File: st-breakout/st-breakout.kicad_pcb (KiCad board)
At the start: 2 copper layers, 72 x 51 mm, 35 parts, among them J1 SPI, J2 SWD, J3 USB4085-GF-A_REVB, J4 USART, SW1 SW_SPDT, U1 AP63203WU, U2 STM32F070F6Px, Y1 16 MHz

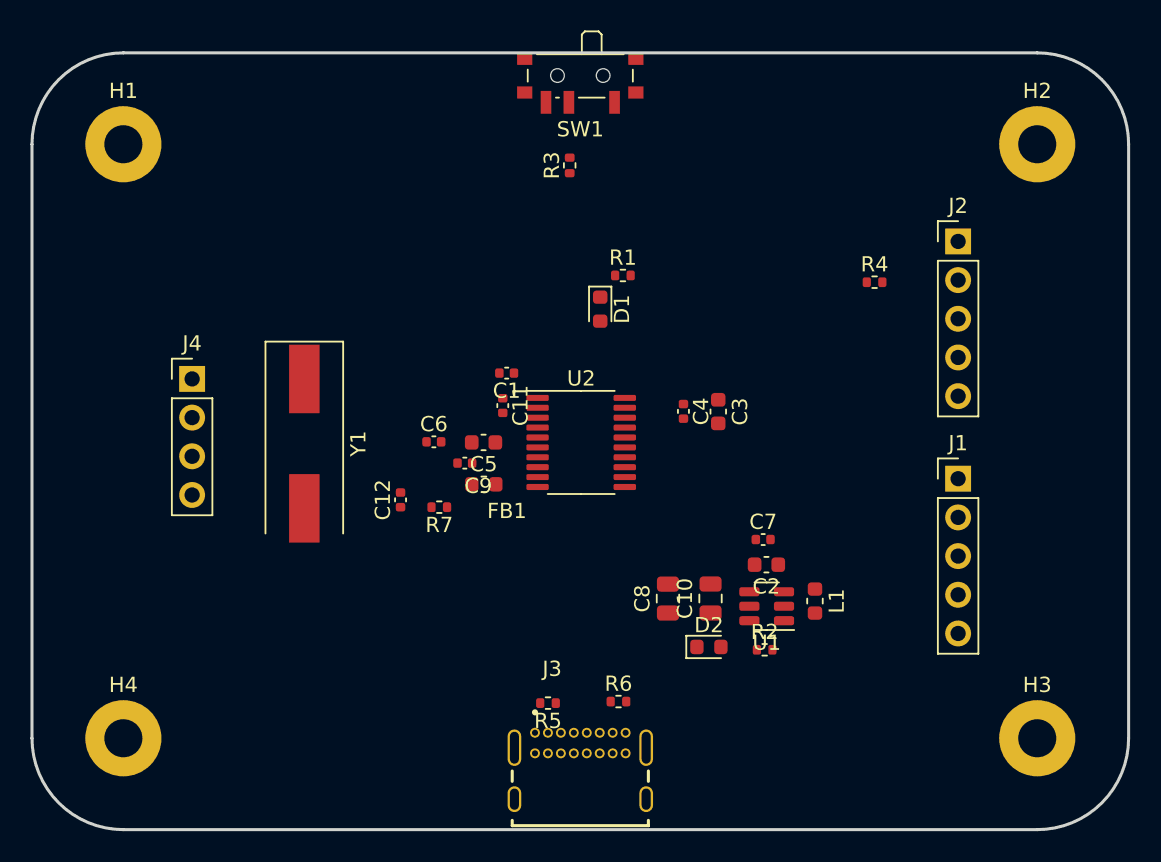
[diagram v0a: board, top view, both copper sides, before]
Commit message: routing and gerber
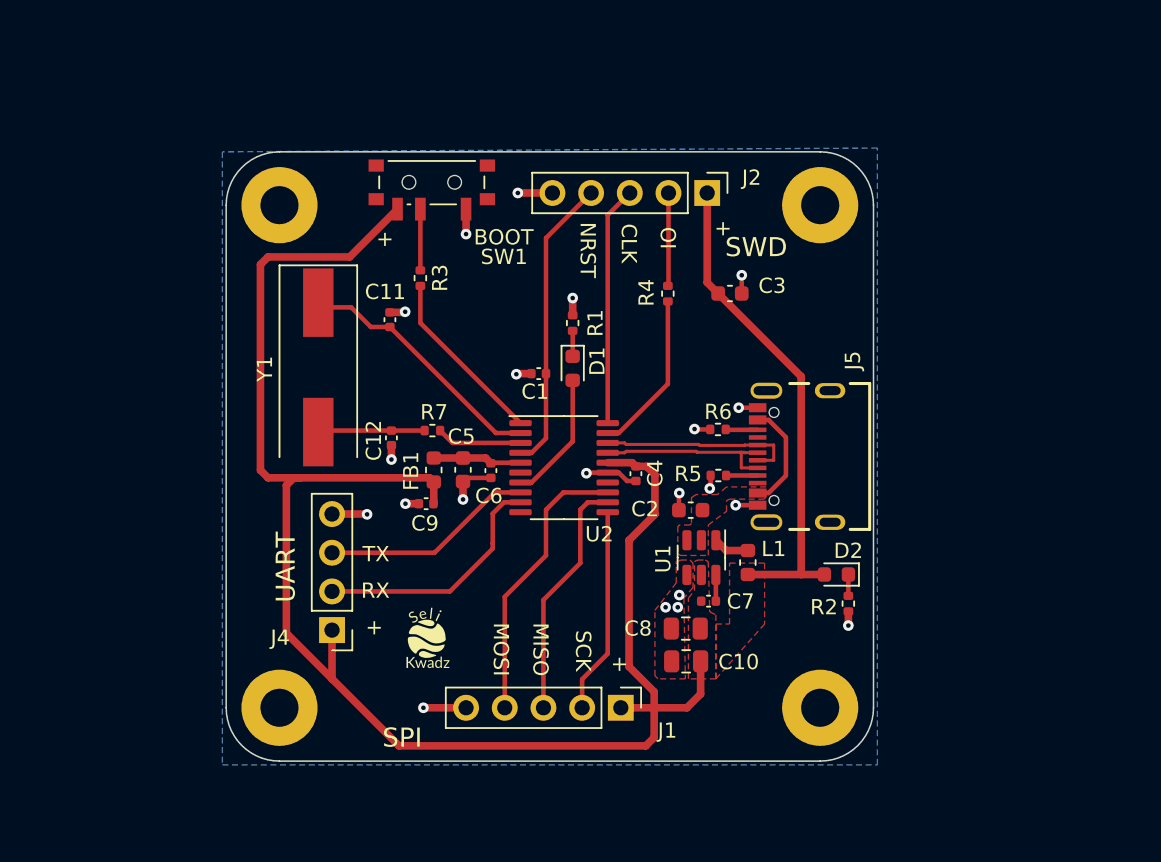
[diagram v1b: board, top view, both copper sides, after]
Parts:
- removed J3: USB4085-GF-A_REVB, USB4085-GF-A:GCT_USB4085-GF-A_REVB
- added G***: LOGO, LOGO, F.Cu at (127.5, 106.4)
- added J5: USB4105-GF-A-060, USB4105-GF-A-060:GCT_USB4105-GF-A-060, F.Cu at (153.9, 94.5)
- moved J1 26.8 mm to (140.2, 111.0), turned to -90 degrees
- moved R6 19.0 mm to (146.5, 92.7)
- moved J4 18.9 mm to (121.2, 105.9), turned to 180 degrees
- moved R5 18.7 mm to (146.6, 95.8), turned to 0 degrees
- moved J2 16.8 mm to (145.8, 77.2), turned to -90 degrees
- moved H2 14.8 mm to (153.2, 78.0)
- moved H3 14.4 mm to (153.2, 111.0)
- moved R4 13.6 mm to (143.2, 83.8), turned to 90 degrees
- moved R3 12.3 mm to (127.0, 82.8)
- moved SW1 12.0 mm to (127.8, 76.8)
- moved H1 11.0 mm to (117.8, 78.0)
- moved H4 10.4 mm to (117.8, 111.0)
- moved D2 9.63 mm to (154.3, 102.2), turned to 180 degrees
- moved C11 9.31 mm to (125.0, 85.5), turned to 90 degrees
- moved C3 7.79 mm to (147.3, 83.8), turned to 0 degrees
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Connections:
- J4 pad 2: USART_TX -> USART_RX
- J4 pad 3: USART_RX -> USART_TX
- R5 pad 1: Net-(J3-CC1) -> GND
- R5 pad 2: GND -> Net-(J5-CC1)
- R6 pad 1: Net-(J3-CC2) -> GND
- R6 pad 2: GND -> Net-(J5-CC2)
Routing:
- net +3.3V: track 0.00 -> 141.0 mm
- net GND: track 0.00 -> 28.5 mm, vias 0 -> 21
- net NRST: track 0.00 -> 19.4 mm
- net SPI_MOSI: track 0.00 -> 18.6 mm
- net HSE_IN: track 0.00 -> 16.7 mm
- net USART_RX: track 0.00 -> 16.1 mm
- net SPI_MISO: track 0.00 -> 16.0 mm
- net SWDCLK: track 0.00 -> 15.7 mm
- net USART_TX: track 0.00 -> 14.0 mm
- net SPI_SCK: track 0.00 -> 13.5 mm
- net USB_D+: track 0.00 -> 13.0 mm
- net USB_D-: track 0.00 -> 12.0 mm
- net BOOT: track 0.00 -> 11.7 mm
- net SWDIO: track 0.00 -> 10.7 mm
- net Net-(D1-A): track 0.00 -> 8.55 mm
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- added copper zone on F.Cu, net +3.3V
- added copper zone on B.Cu, net GND
- added copper zone on F.Cu, net GND
- added copper zone on F.Cu, net VBUS
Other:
- board size 72 x 51 mm -> 42.5 x 40 mm
- rule pad_to_mask_clearance: 0 -> 0.0508
- board text added: "+"
- board text added: "6/10/2023 V1.0"
- board text added: "BOOT"
- board text added: "CLK"
- board text added: "IO"
- board text added: "MISO"
- board text added: "MOSI"
- board text added: "NRST"
- board text added: "RX"
- board text added: "SCK"
- board text added: "SPI"
- board text added: "SWD"
- board text added: "TX"
- board text added: "UART"
